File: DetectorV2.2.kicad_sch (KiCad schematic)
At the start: 27 parts, among them J1 Conn_01x02, SW2 SW_SPST, U1 AD8092ARZ-REEL7

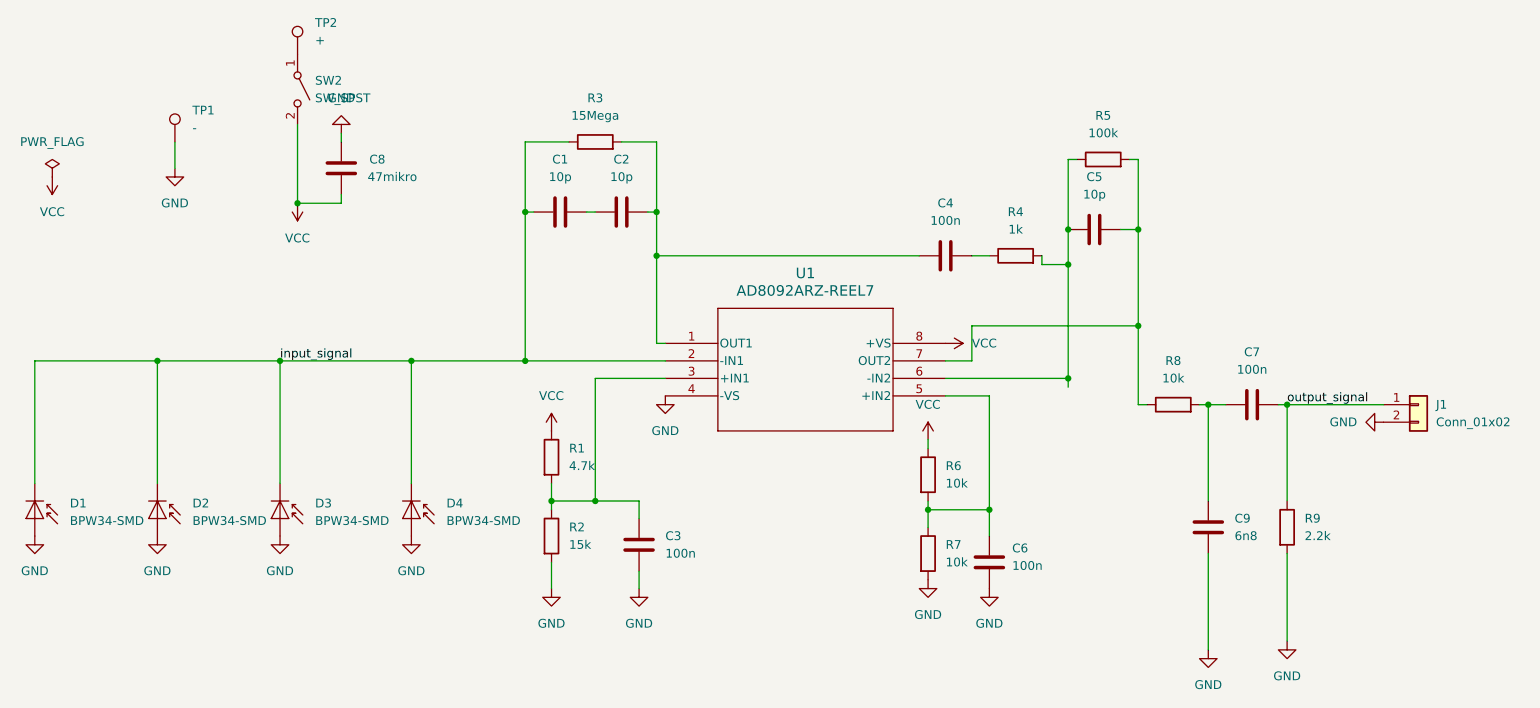
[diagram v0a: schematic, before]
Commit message: updated
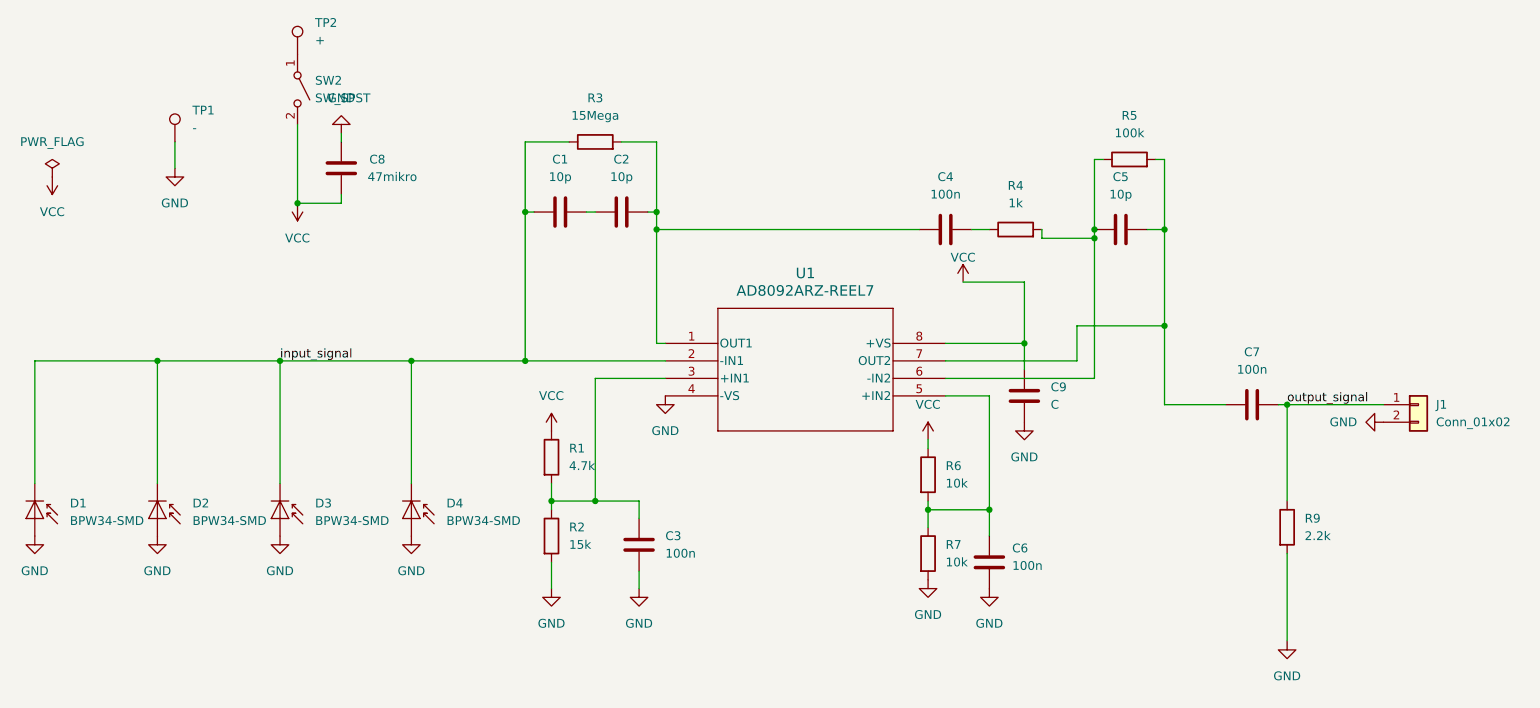
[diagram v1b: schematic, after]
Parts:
- removed R8: 10k, Resistor_SMD:R_0805_2012Metric, symbol Device:R
- C9: value 6n8 -> C; footprint Capacitor_SMD:C_0805_2012Metric -> (none)
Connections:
- net VCC: now also C9.1
- net at C5.2, R5.2, U1.7 (OUT2): now also C7.1
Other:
- moved on the sheet: C4, C5, R4, R5
